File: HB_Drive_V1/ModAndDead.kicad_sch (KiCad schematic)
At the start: 24 parts, among them J401 Conn_01x02, J402 Conn_01x02, U401 LM311, U402 74LS08, U403 74AUC2G02, U404 74LS365

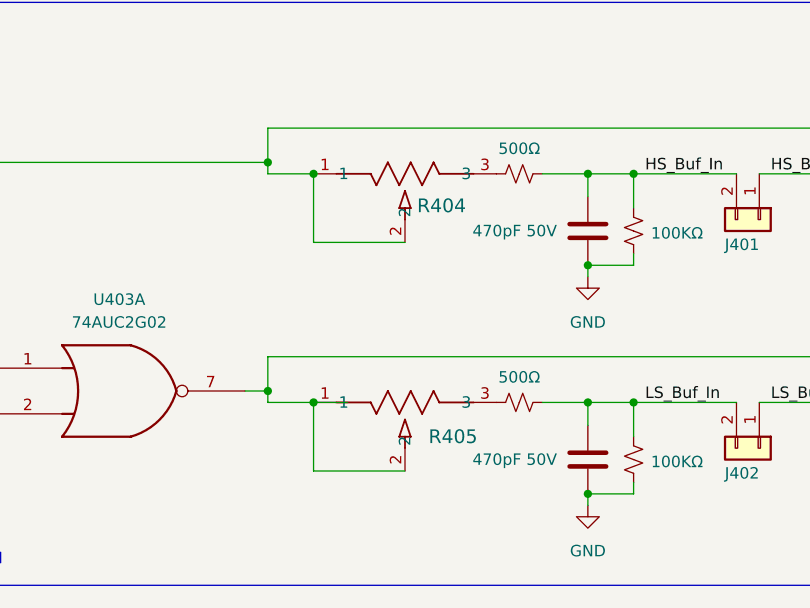
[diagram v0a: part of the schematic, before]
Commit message: commits latest kiCAD project for BOM generation
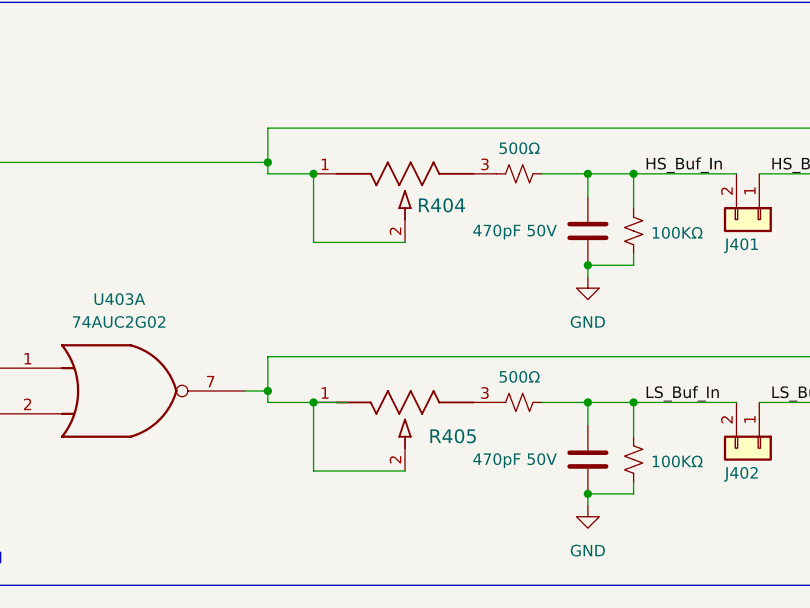
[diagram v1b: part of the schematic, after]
